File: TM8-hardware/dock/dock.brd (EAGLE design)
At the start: 37.5 x 55 mm, 0 parts

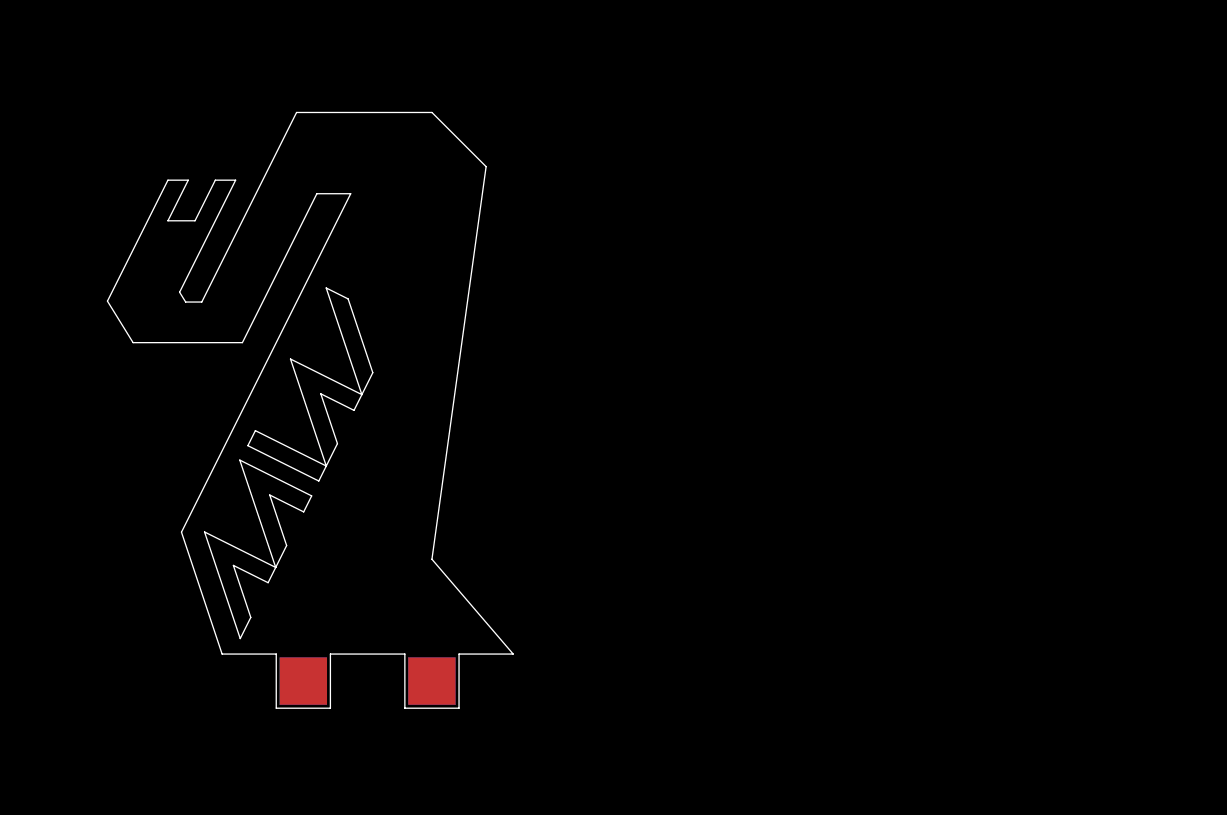
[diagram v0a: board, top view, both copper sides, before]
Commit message: updated with more stuff
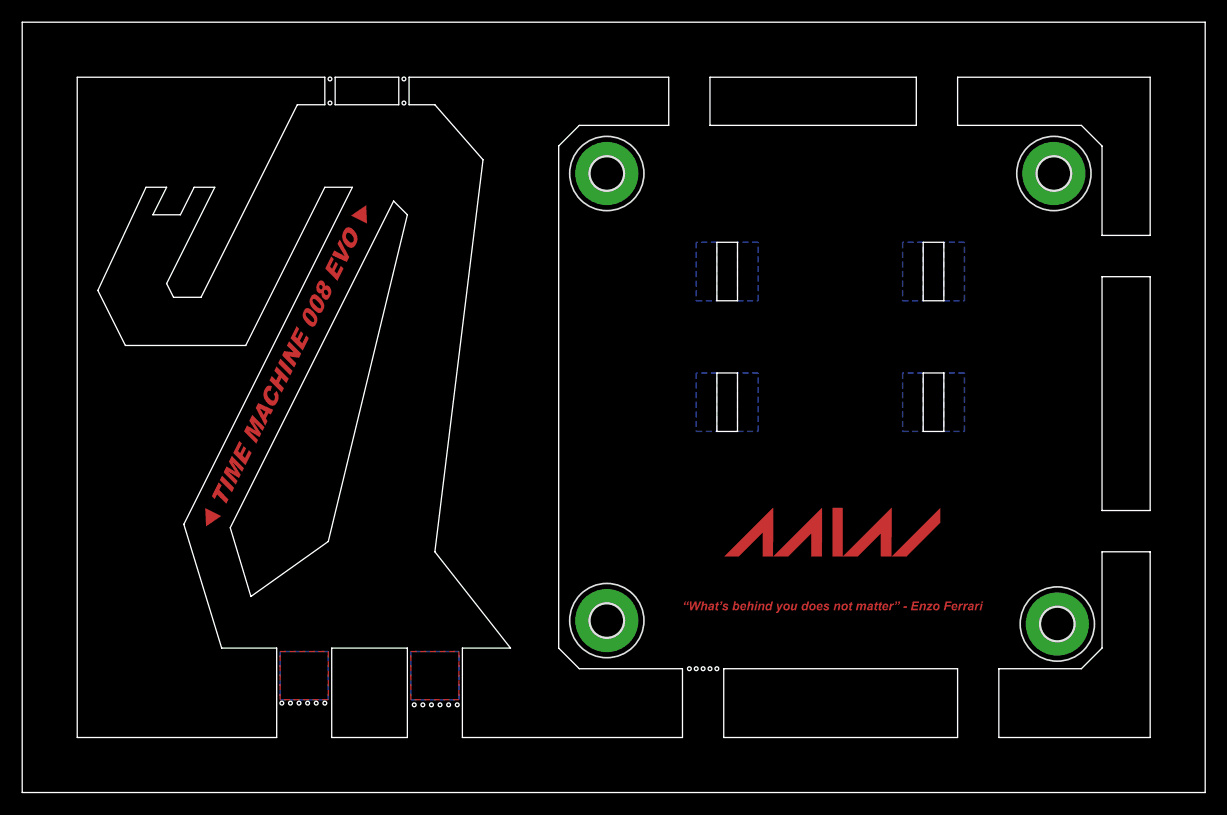
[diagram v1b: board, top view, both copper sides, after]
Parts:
- added H1, H2, H3, H4: MOUNT-PAD-ROUND3.0, holes:3,0-PAD
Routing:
- added copper zone on layer 1, net PAD
- added copper zone on layer 16, net PAD
- added copper zone on layer 16, net PAD1
- added copper zone on layer 16, net PAD10
- added copper zone on layer 1, net PAD2
- added copper zone on layer 16, net PAD3
- added copper zone on layer 16, net PAD4
- added copper zone on layer 16, net PAD5
- added copper zone on layer 16, net PAD6
- added copper zone on layer 16, net PAD7
- added copper zone on layer 16, net PAD8
- added copper zone on layer 16, net PAD9
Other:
- board size 37.5 x 55 mm -> 109.2 x 71.1 mm
